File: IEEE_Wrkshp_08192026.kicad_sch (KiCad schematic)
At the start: 26 parts, among them J1 Screw_Terminal_01x03, J2 Screw_Terminal_01x02, Q1 RS9N50D, T1 Transformer_1P_1S, U1 Opamp_Dual

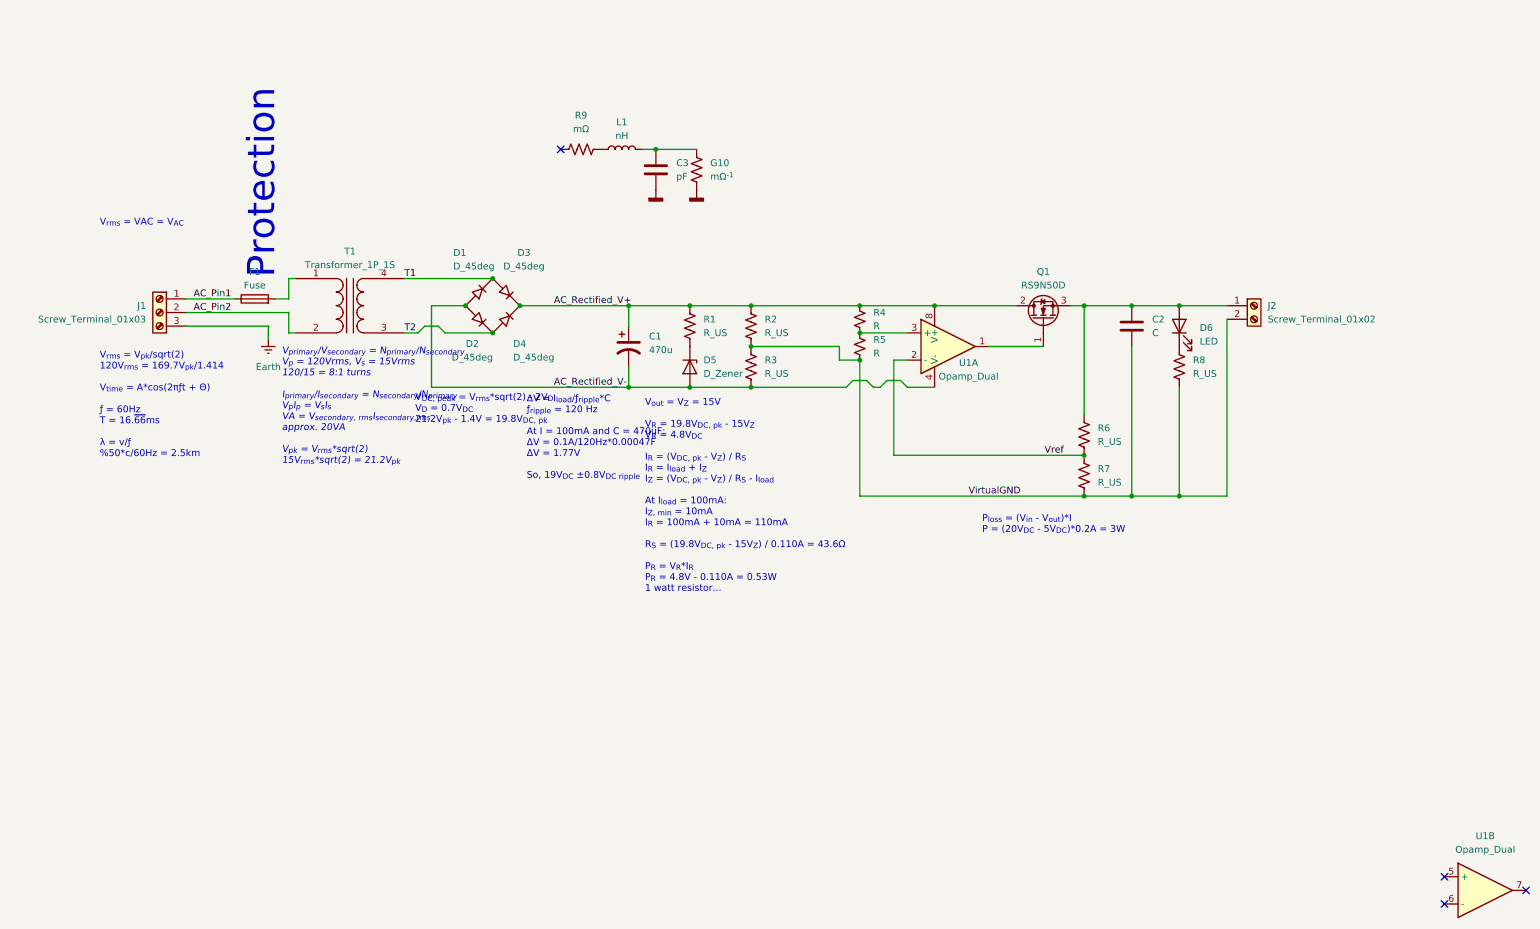
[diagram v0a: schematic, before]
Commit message: Testing commit
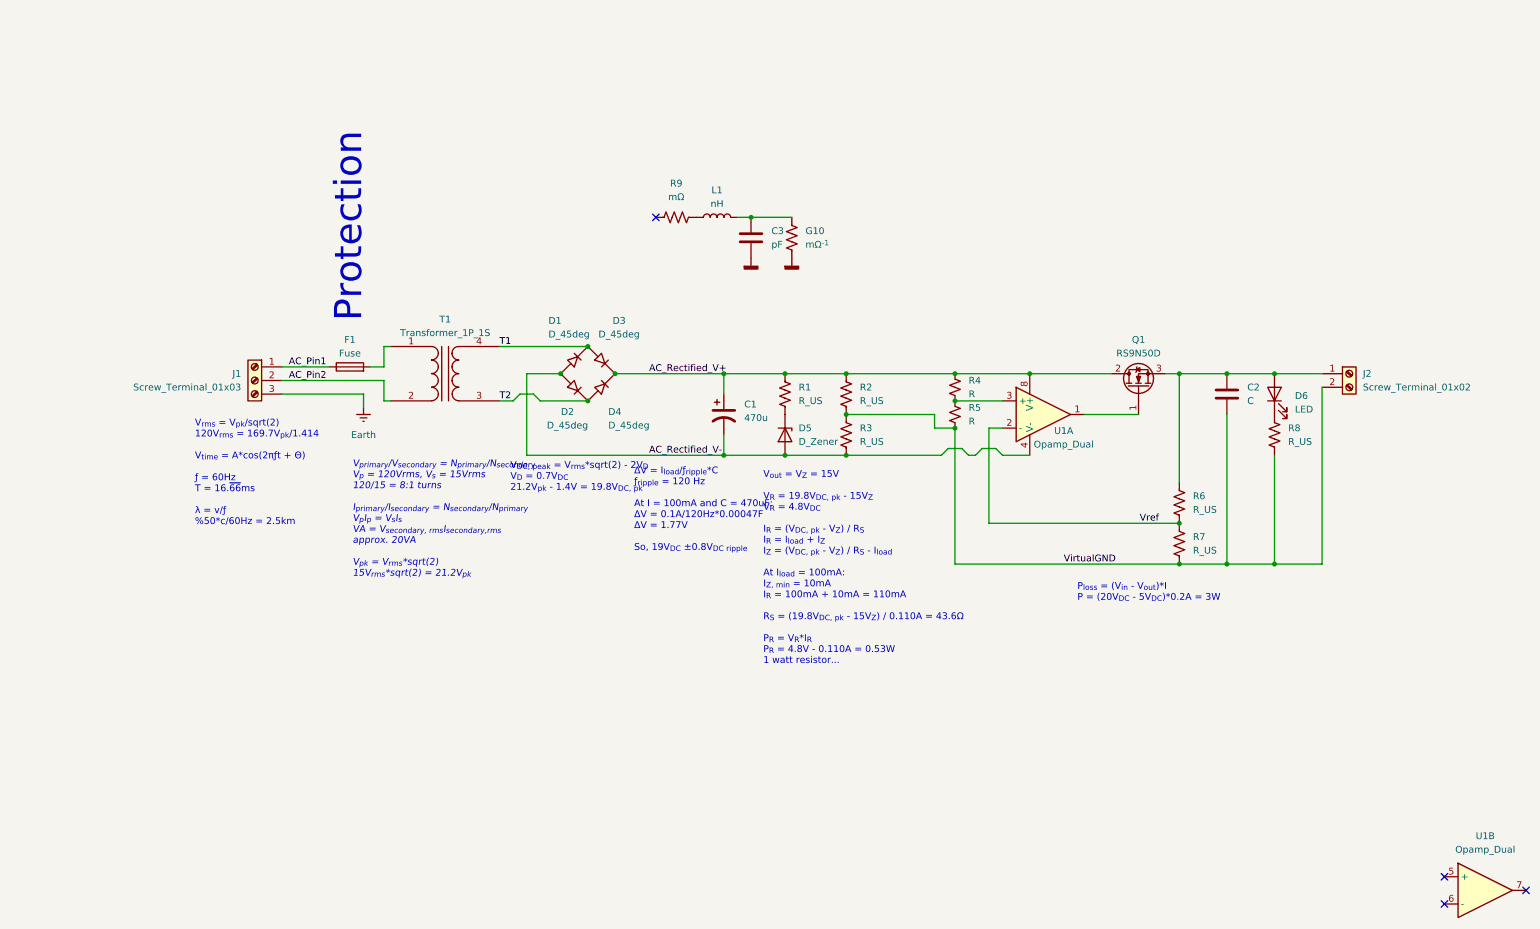
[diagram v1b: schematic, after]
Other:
- note removed: "V_{rms} = VAC = V_{AC}"
- moved on the sheet: C1, C2, C3, D1, D2, D3, D4, D5, D6, F1, G10, J1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
